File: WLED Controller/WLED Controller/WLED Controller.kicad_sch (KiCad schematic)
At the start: 2 parts, among them U1 ESP32-WROOM-32, U2 SN74AHCT125N

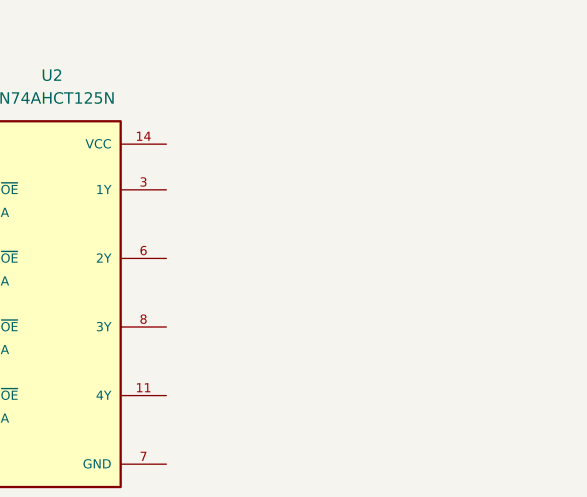
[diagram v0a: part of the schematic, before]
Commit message: Audio Jack Added
Added Audio Jack
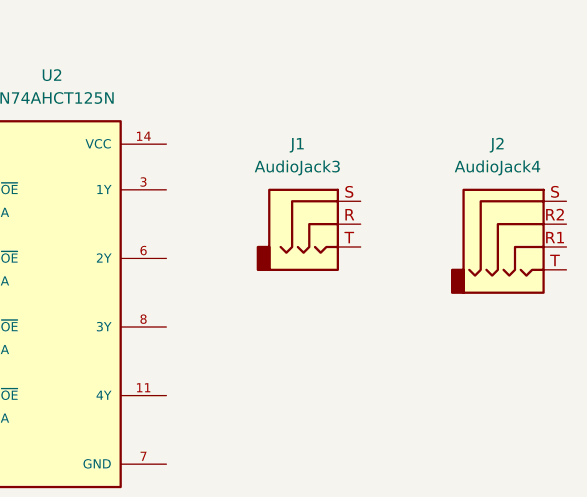
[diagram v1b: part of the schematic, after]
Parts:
- added J1: AudioJack3, Connector_Audio:Jack_3.5mm_CUI_SJ-3523-SMT_Horizontal, symbol Connector_Audio:AudioJack3
- added J2: AudioJack4, Connector_Audio:Jack_3.5mm_PJ320D_Horizontal, symbol Connector_Audio:AudioJack4
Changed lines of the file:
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@@
+	)
+	(symbol
+		(lib_id "Connector_Audio:AudioJack4")
+		(at 218.44 55.88 0)
+		(unit 1)
+		(exclude_from_sim no)
+		(in_bom yes)
+		(on_board yes)
+		(dnp no)
+		(fields_autoplaced yes)
+		(property "Reference" "J2"
+			(at 215.9 46.99 0)
+			(effects
+				(font
+					(size 1.27 1.27)
+				)
+			)
+		)
+		(property "Value" "AudioJack4"
+			(at 215.9 49.53 0)
+			(effects
+				(font
+					(size 1.27 1.27)
+				)
+			)
+		)
+		(property "Footprint" "Connector_Audio:Jack_3.5mm_PJ320D_Horizontal"
+			(at 218.44 55.88 0)
+			(effects
+				(font
+					(size 1.27 1.27)
+				)
+				(hide yes)
+			)
+		)
+		(property "Datasheet" "https://sharvielectronics.com/wp-content/uploads/2021/07/Audio-Jack-3.5mm-TRRS-SMD.pdf"
+			(at 218.44 55.88 0)
+			(effects
+				(font
+					(size 1.27 1.27)
+				)
+				(hide yes)
+			)
+		)
+		(property "Description" "Audio Jack, 4 Poles (TRRS)"
+			(at 218.44 55.88 0)
+			(effects
+				(font
+					(size 1.27 1.27)
+				)
+				(hide yes)
+			)
+		)
+		(pin "S"
+		)
+		(pin "R2"
+		)
+		(pin "R1"
+		)
+		(pin "T"
+		)
+		(instances
+			(project ""
+				(path "/e8736a94-4ef8-408c-b7cc-dcf1b7df2117"
+					(reference "J2")
+					(unit 1)
+				)
+			)
+		)
 	)
 	(symbol
@@
 					(unit 1)
 				)
+			)
+		)
+	)
+	(symbol
+		(lib_id "Connector_Audio:AudioJack3")
+		(at 195.58 55.88 0)
+		(unit 1)
+		(exclude_from_sim no)
+		(in_bom yes)
+		(on_board yes)
+		(dnp no)
+		(fields_autoplaced yes)
+		(property "Reference" "J1"
+			(at 193.675 46.99 0)
+			(effects
+				(font
+					(size 1.27 1.27)
+				)
+			)
+		)
+		(property "Value" "AudioJack3"
+			(at 193.675 49.53 0)
+			(effects
+				(font
+					(size 1.27 1.27)
+				)
+			)
+		)
+		(property "Footprint" "Connector_Audio:Jack_3.5mm_CUI_SJ-3523-SMT_Horizontal"
+			(at 195.58 55.88 0)
+			(effects
+				(font
+					(size 1.27 1.27)
+				)
+				(hide yes)
+			)
+		)
+		(property "Datasheet" "~"
+			(at 195.58 55.88 0)
+			(effects
+				(font
+					(size 1.27 1.27)
+				)
+				(hide yes)
+			)
+		)
+		(property "Description" "Audio Jack, 3 Poles (Stereo / TRS)"
+			(at 195.58 55.88 0)
+			(effects
+				(font
+					(size 1.27 1.27)
+				)
+				(hide yes)
+			)
+		)
+		(pin "R"
+		)
+		(pin "S"
+		)
+		(pin "T"
+		)
+		(instances
+			(project ""
+				(path "/e8736a94-4ef8-408c-b7cc-dcf1b7df2117"
+					(reference "J1")
+					(unit 1)
+				)

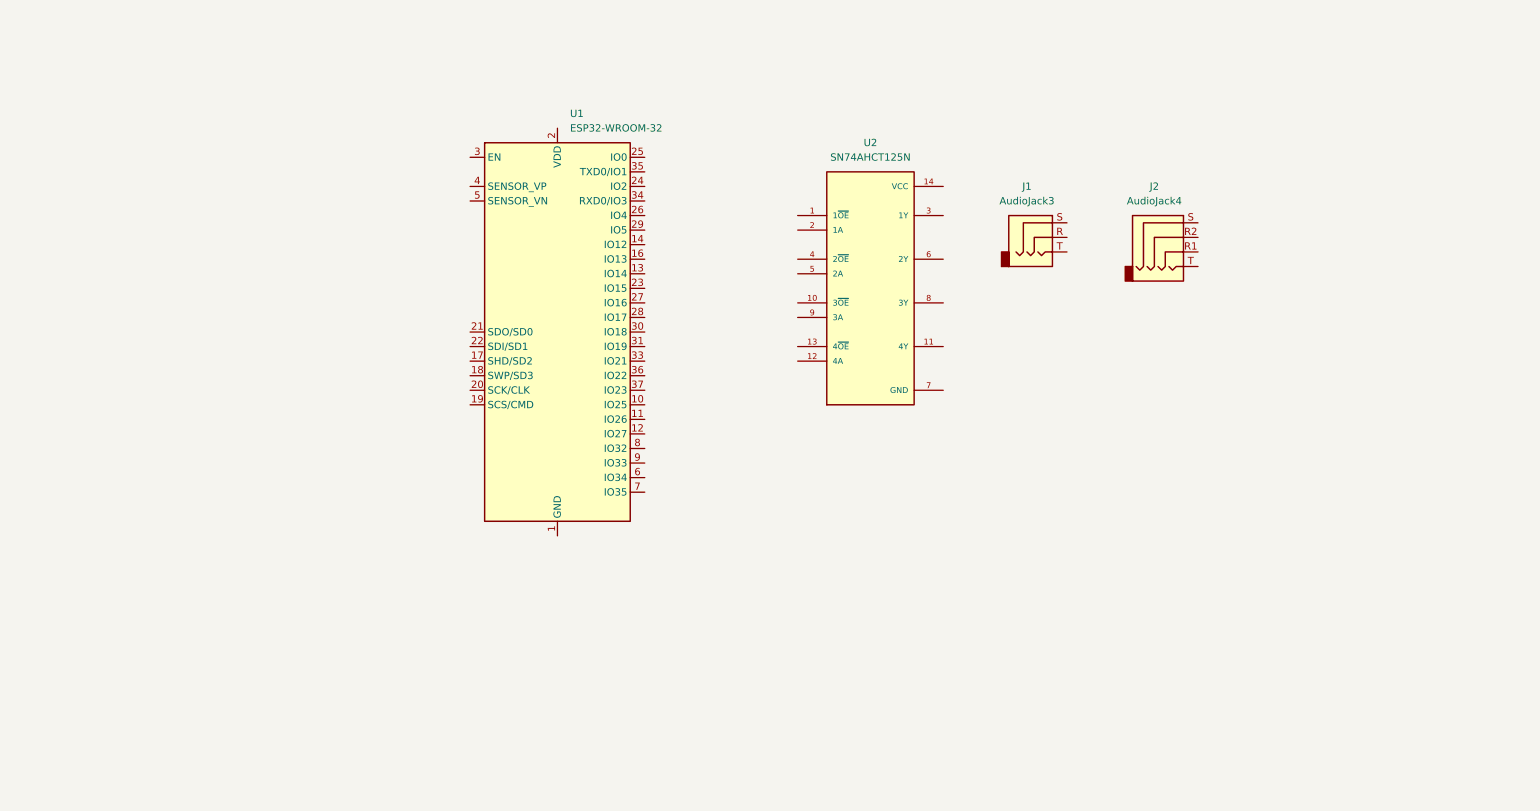
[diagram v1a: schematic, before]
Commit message: ADDED
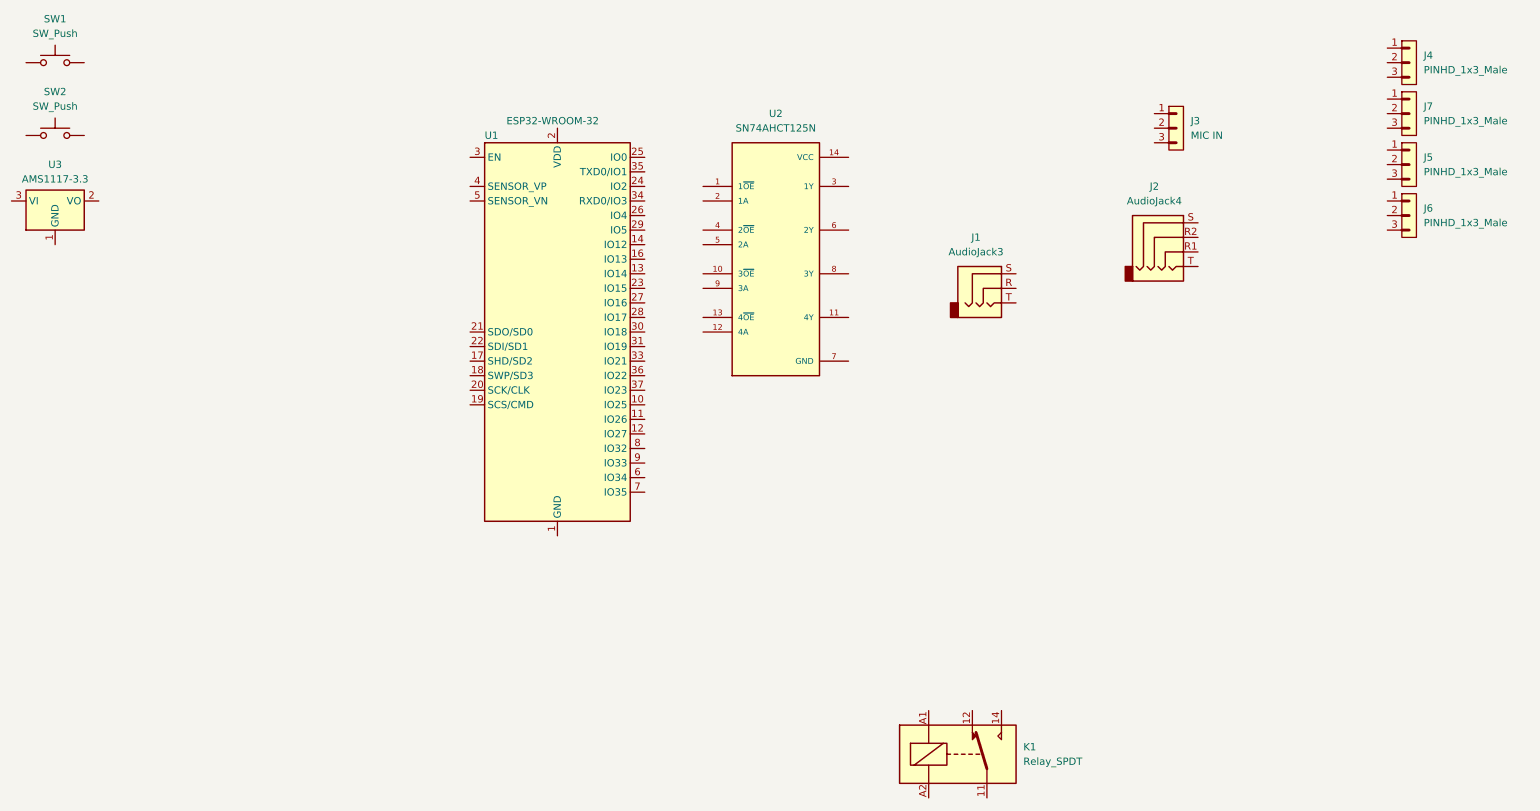
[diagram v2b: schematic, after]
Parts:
- added J3: MIC IN, Connector_PinHeader_2.54mm:PinHeader_1x03_P2.54mm_Vertical, symbol PCM_SL_Pin_Headers:PINHD_1x3_Male
- added J4, J5, J6, J7: PINHD_1x3_Male, Connector_PinHeader_2.54mm:PinHeader_1x03_P2.54mm_Vertical, symbol PCM_SL_Pin_Headers:PINHD_1x3_Male
- added K1: Relay_SPDT, symbol Relay:Relay_SPDT
- added SW1, SW2: SW_Push, symbol Switch:SW_Push
- added U3: AMS1117-3.3, Package_TO_SOT_SMD:SOT-223-3_TabPin2, symbol Regulator_Linear:AMS1117-3.3
- U1: Design Guide (none) -> file:///C:/Users/ARUN/Desktop/COMPS/ESP32-WROOM-32E_V1.2_Re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
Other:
- moved on the sheet: J1, U2
